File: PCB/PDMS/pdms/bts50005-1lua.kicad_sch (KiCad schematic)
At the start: 11 parts, among them Q3 BTS500101LUAAUMA1

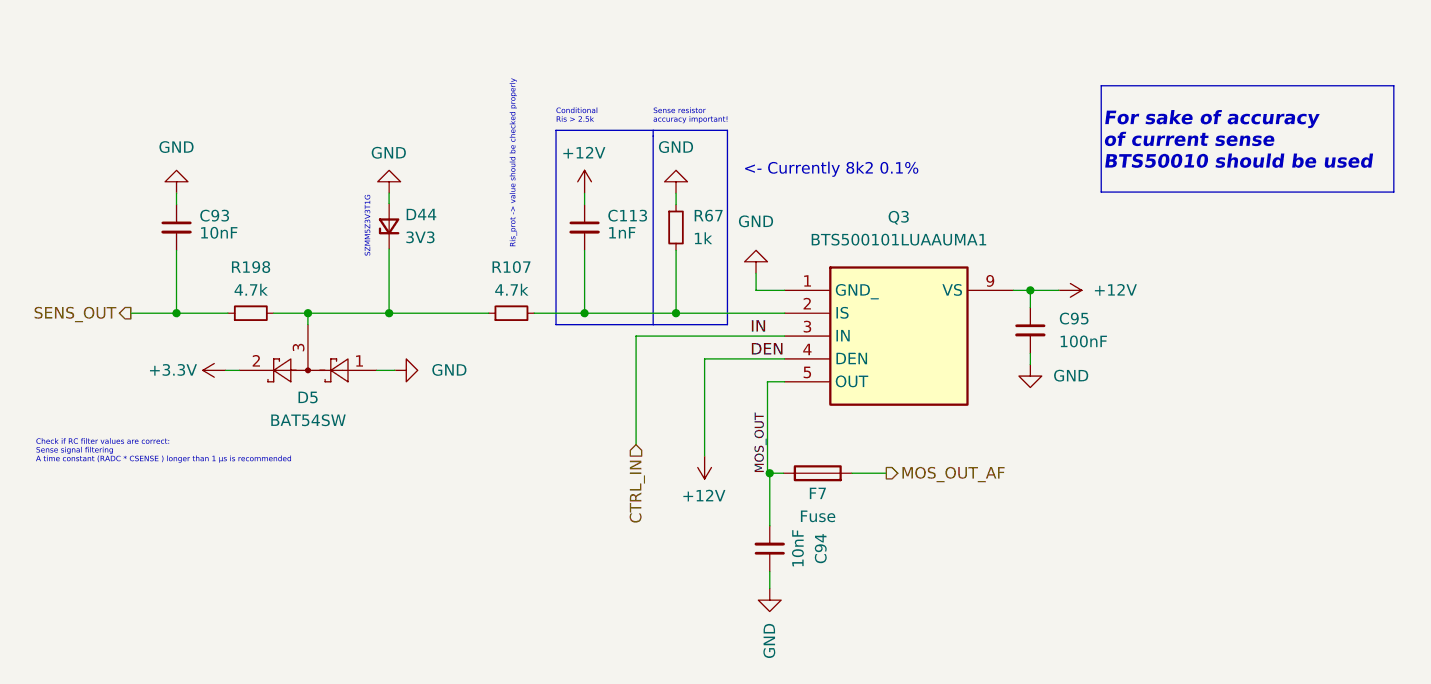
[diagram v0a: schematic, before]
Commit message: PDMS PCB input modification WIP - no supply
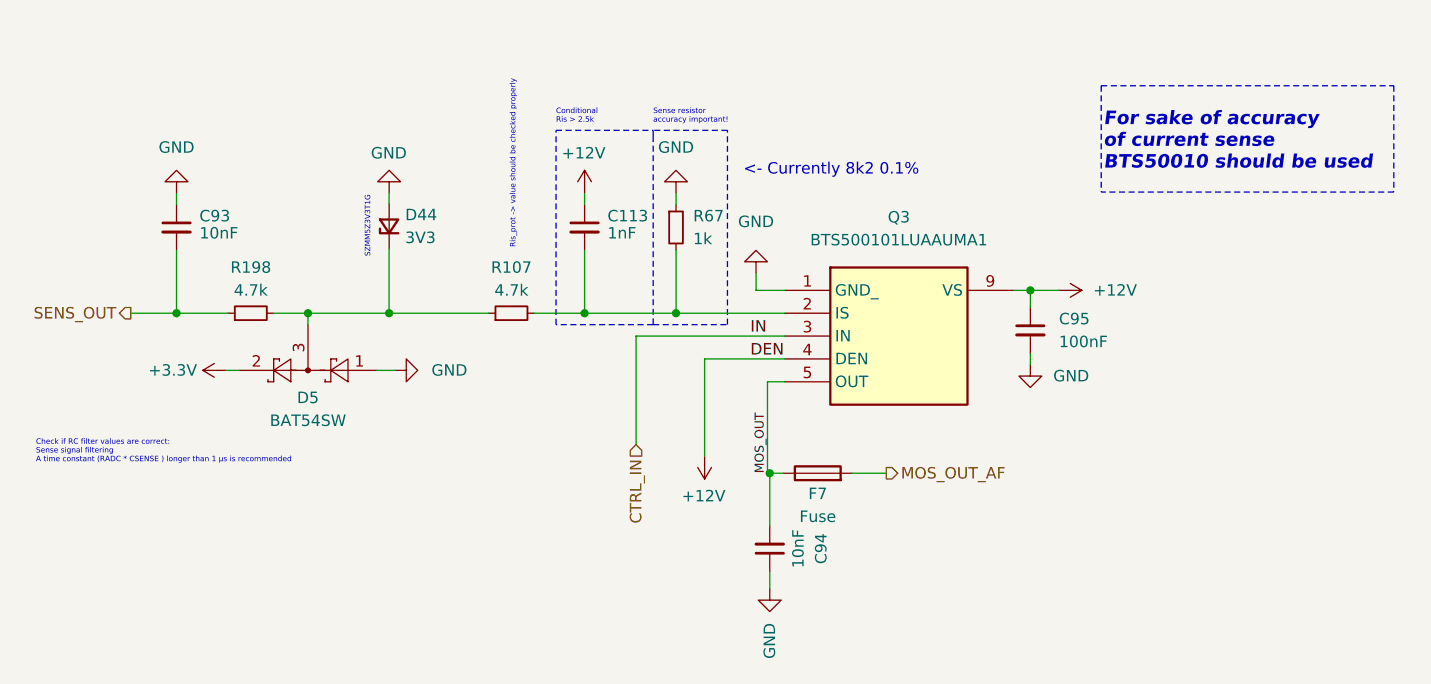
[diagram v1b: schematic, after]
